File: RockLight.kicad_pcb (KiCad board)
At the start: 2 copper layers, 47 x 53 mm, 18 parts, among them J1 USB_C_Receptacle_USB2.0_16P, J2 ISP, SW1 USER, SW2 RESET, U1 ATtiny85-10SU

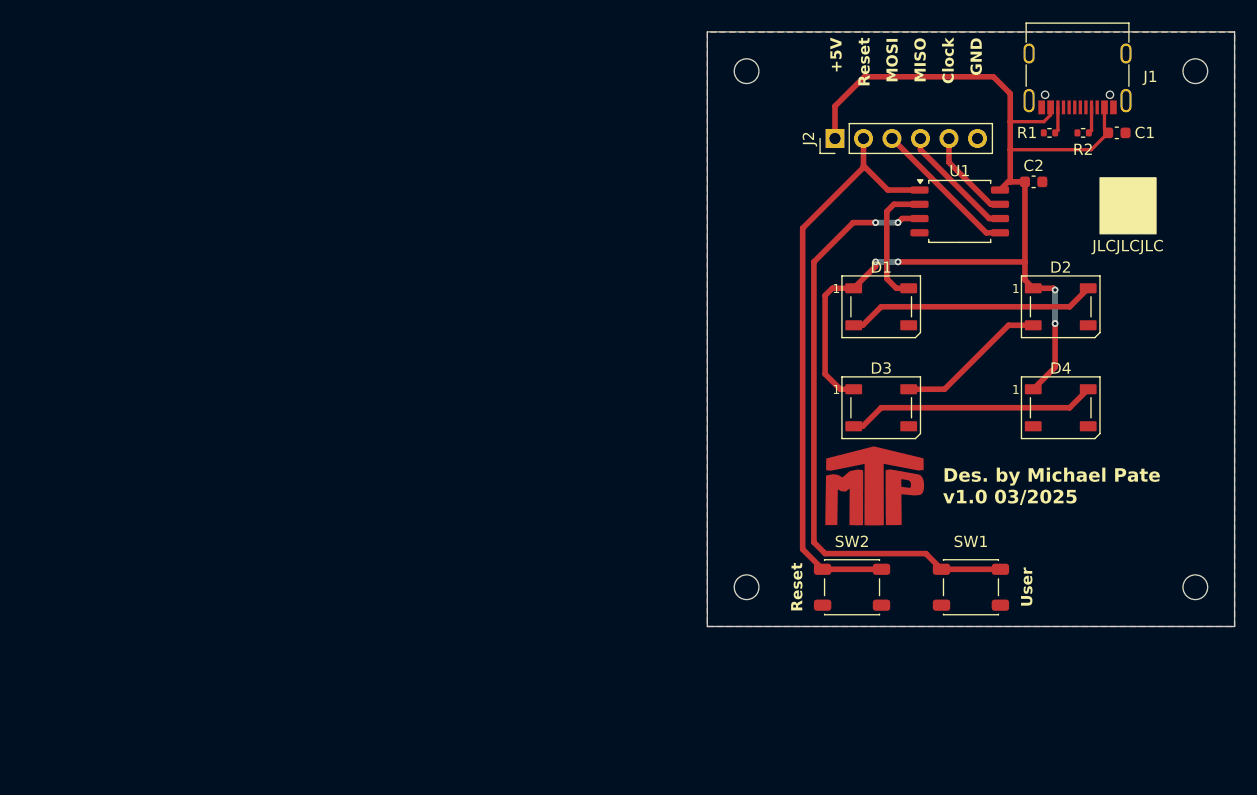
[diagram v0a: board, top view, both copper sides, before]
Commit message: Add project files
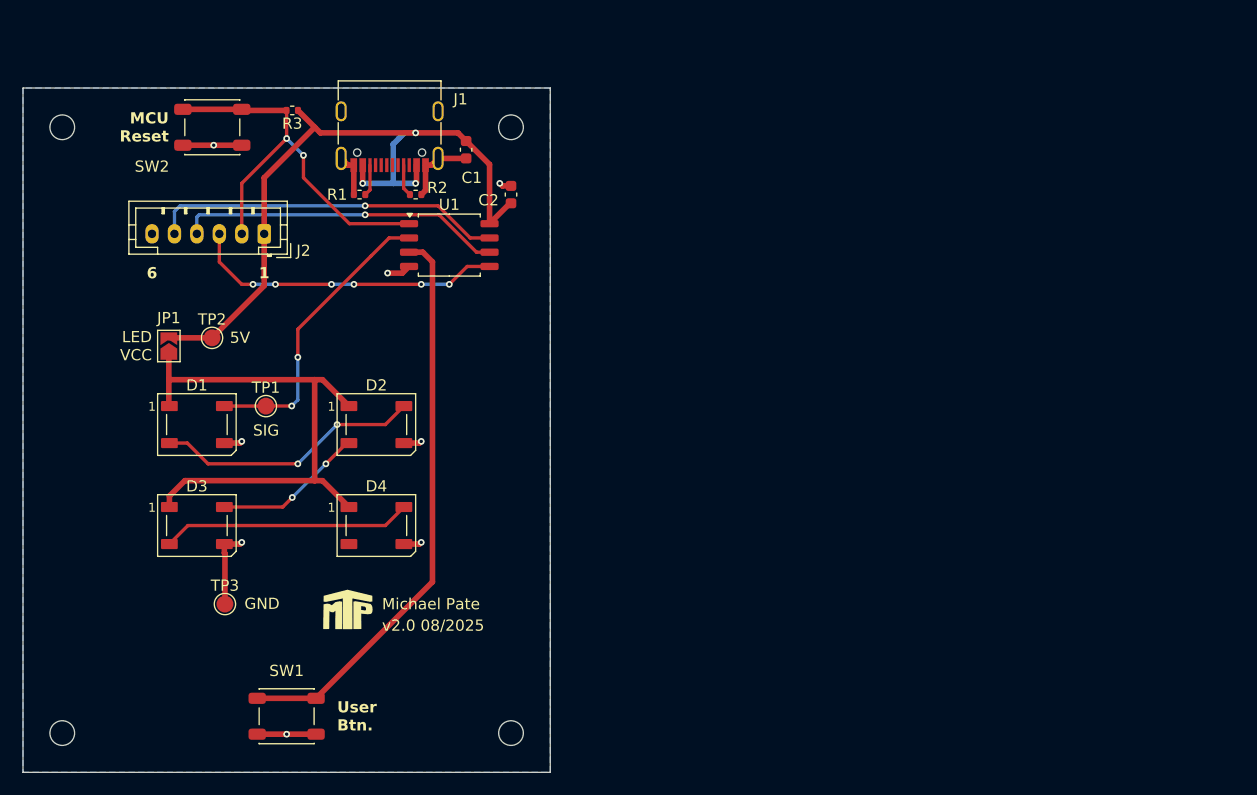
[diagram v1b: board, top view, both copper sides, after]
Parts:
- removed the REF** at (214.0, 82.5)
- added JP1: Jumper_2_Small_Open, Jumper:SolderJumper-2_P1.3mm_Open_TrianglePad1.0x1.5mm, F.Cu at (151.0, 70.0)
- added R3: 10k, Resistor_SMD:R_0402_1005Metric, F.Cu at (162.0, 49.0)
- added REF**: MTP Logo 5mm Low Detail, Watermarks:MTP Logo 5mm Low Detail, F.Cu at (167.0, 94.0)
- added TP1: SIG, TestPoint:TestPoint_Pad_D1.5mm, F.Cu at (159.7, 75.4)
- added TP2: +5V, TestPoint:TestPoint_Pad_D1.5mm, F.Cu at (154.9, 69.3)
- added TP3: GND, TestPoint:TestPoint_Pad_D1.5mm, F.Cu at (156.0, 93.0)
- J2: footprint Connector_PinHeader_2.54mm:PinHeader_1x06_P2.54mm_Vertical -> Connector_JST:JST_PH_B6B-PH-K_1x06_P2.00mm_Vertical
- moved SW2 70.2 mm to (154.9, 50.5)
- moved H3 62.4 mm to (141.5, 104.5)
- moved H4 62.4 mm to (181.5, 104.5)
- moved SW1 62.1 mm to (161.5, 103.0)
- moved D1 61.9 mm to (153.5, 77.0)
- moved D2 61.9 mm to (169.5, 77.0)
- moved D3 61.9 mm to (153.5, 86.0)
- moved D4 61.9 mm to (169.5, 86.0)
- moved R1 61.7 mm to (168.0, 56.5)
- moved J1 61.5 mm to (170.7, 50.1)
- moved H1 61.2 mm to (141.5, 50.5)
- moved H2 61.2 mm to (181.5, 50.5)
- moved R2 59.8 mm to (173.0, 56.5), turned to 180 degrees
- moved C1 58.0 mm to (177.5, 52.5), turned to -90 degrees
- moved J2 51.6 mm to (159.5, 60.0), turned to 180 degrees
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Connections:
- D1 pad 1: +5V -> Net-(D1-VDD)
- D2 pad 1: +5V -> Net-(D1-VDD)
- D3 pad 1: +5V -> Net-(D1-VDD)
- D4 pad 1: +5V -> Net-(D1-VDD)
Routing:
- net Net-(D1-VDD): track 0.00 -> 49.2 mm
- net GND: track 0.00 -> 36.2 mm, vias 0 -> 8
- net +5V: track 97.7 -> 67.4 mm, vias 4 -> 3
- net /SCK: track 8.23 -> 31.5 mm, vias 0 -> 1
- net /MISO: track 10.6 -> 29.1 mm, vias 0 -> 1
- net /RESET: track 52.5 -> 37.2 mm, vias 0 -> 2
- net /MOSI: track 13.1 -> 28.1 mm, vias 0 -> 6
- net Net-(D1-DIN): track 11.5 -> 26.4 mm, vias 0 -> 2
- net Net-(SW1-A): track 53.6 -> 50.9 mm, vias 2 -> 0
- net Net-(D1-DOUT): track 22.3 -> 23.8 mm, vias 0 -> 2
- net Net-(D2-DOUT): vias 0 -> 2
- removed copper zone on F.Cu, net GND
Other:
- board size 47 x 53 mm -> 47 x 61 mm
- board text added: "1"
- board text added: "5V"
- board text added: "6"
- board text added: "ISP Connector 1. 5V 2. Reset 3. MOSI 4. MISO 5. Clock 6. GND"
- board text added: "LED VCC"
- board text added: "MCU Reset"
- board text added: "Michael Pate"
- board text added: "SIG"
- board text added: "User Btn."
- board text added: "v2.0 08/2025"
- board text removed: "+5V"
- board text removed: "Clock"
- board text removed: "Des. by Michael Pate v1.0 03/2025"
- board text removed: "JLCJLCJLC"
- board text removed: "MISO"
- board text removed: "MOSI"
- board text removed: "Reset"
- board text removed: "User"
